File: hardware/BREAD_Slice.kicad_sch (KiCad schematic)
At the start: 15 parts, among them J1 Conn_01x10_Female, U1 AP63205

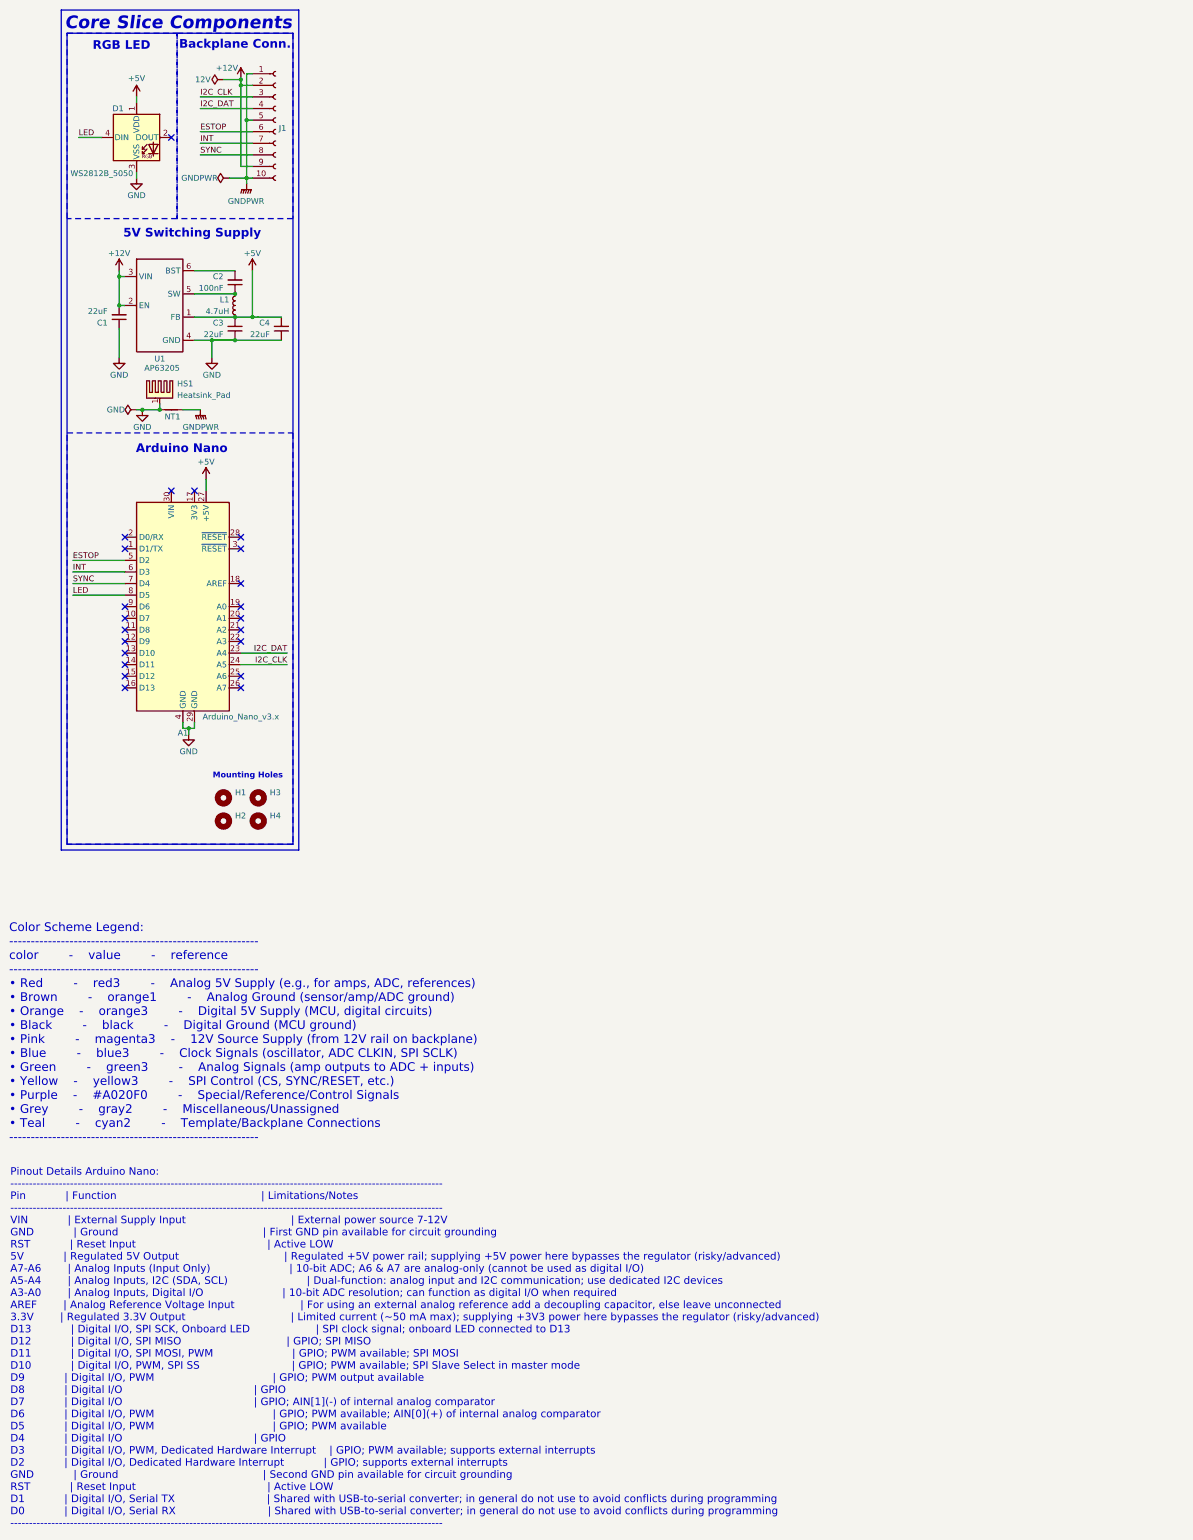
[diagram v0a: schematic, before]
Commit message: initial commit post-fork to r2
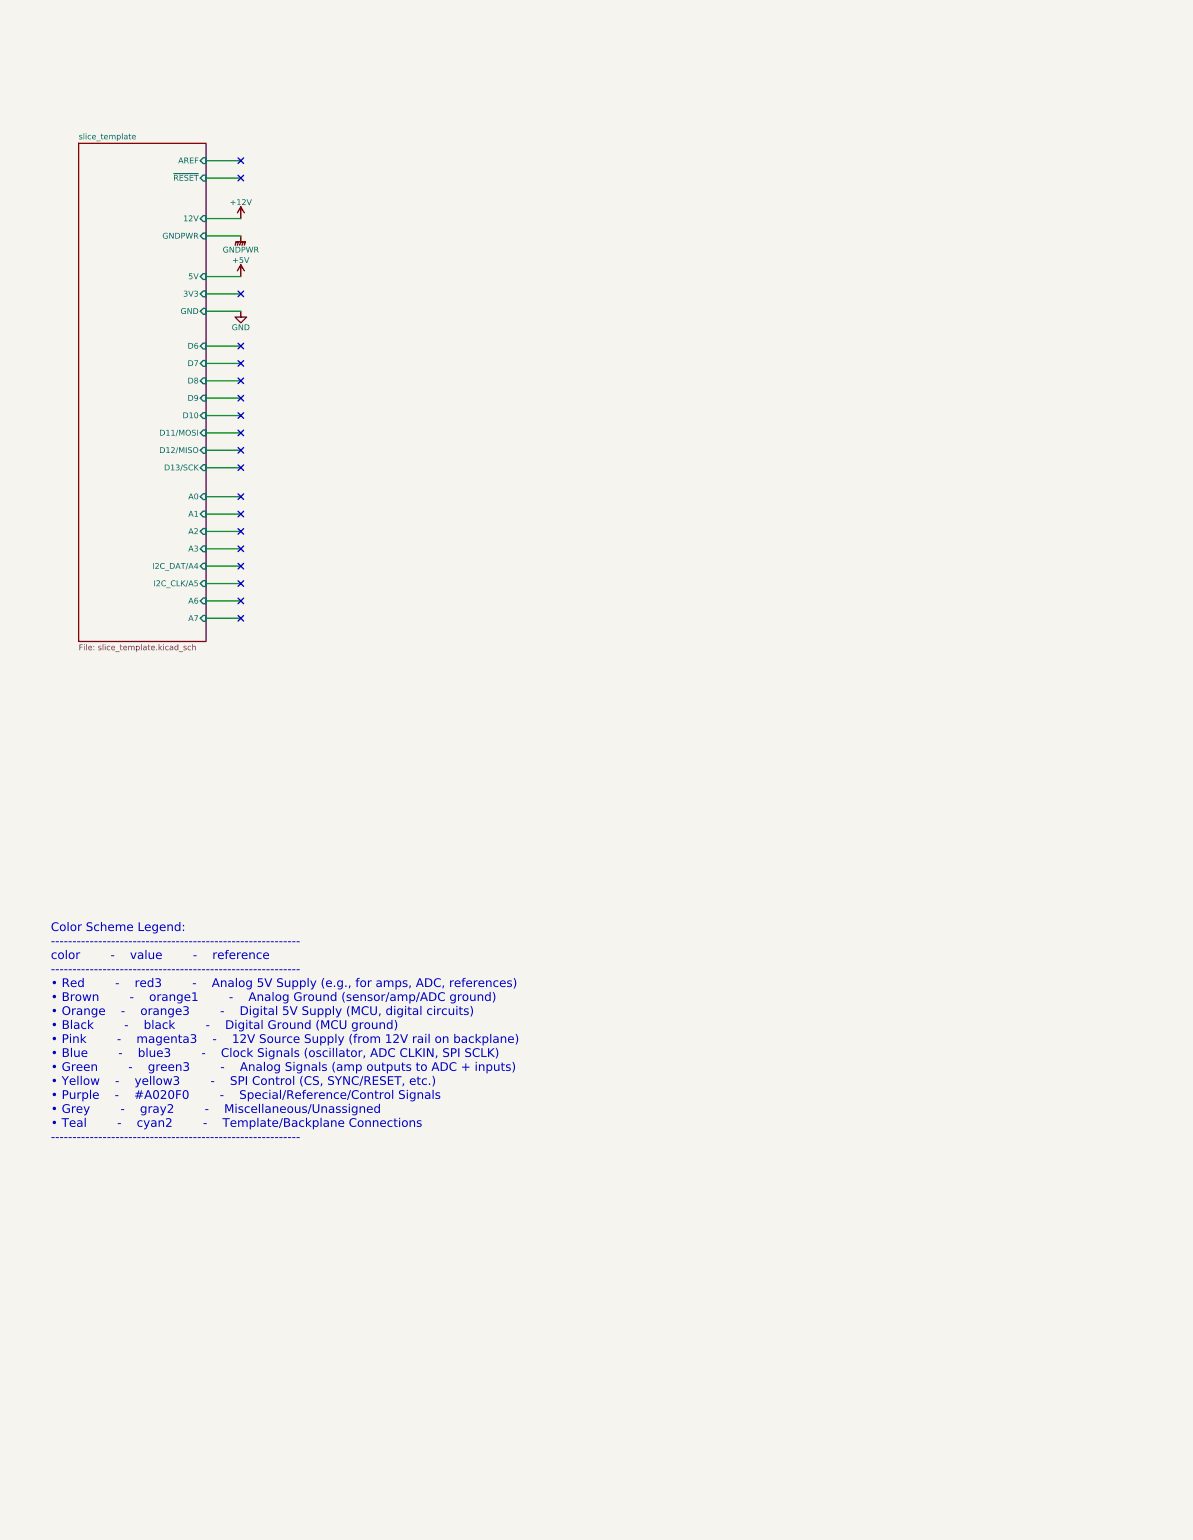
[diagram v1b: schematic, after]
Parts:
- removed A1: Arduino_Nano_v3.x, Module:Arduino_Nano, symbol MCU_Module:Arduino_Nano_v3.x
- removed C1, C3, C4: 22uF, Capacitor_SMD:C_1206_3216Metric, symbol Device:C_Small
- removed C2: 100nF, Capacitor_SMD:C_1206_3216Metric, symbol Device:C_Small
- removed D1: WS2812B_5050, SparkFun-LED:WS2812-5050-4PIN, symbol SparkFun-LED:WS2812B_5050
- removed H1, H2, H3, H4: MountingHole, MountingHole:MountingHole_5mm, symbol Mechanical:MountingHole
- removed HS1: Heatsink_Pad, kml-custom:Thermal Pad, symbol Mechanical:Heatsink_Pad
- removed J1: Conn_01x10_Female, Connector_PinSocket_2.54mm:PinSocket_1x10_P2.54mm_Horizontal, symbol Connector:Conn_01x10_Female
- removed L1: 4.7uH, Inductor_SMD:L_1210_3225Metric, symbol Device:L_Small
- removed NT1: NetTie_2, NetTie:NetTie-2_SMD_Pad2.0mm, symbol Device:NetTie_2
- removed U1: AP63205, Package_TO_SOT_SMD:TSOT-23-6, symbol SparkFun-DiscreteSemi:AP63205
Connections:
- no-connect marks 22 -> 19
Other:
- added sheet slice_template (slice_template.kicad_sch)
- note removed: "5V Switching Supply"
- note removed: "Arduino Nano"
- note removed: "Backplane Conn."
- note removed: "Core Slice Components"
- note removed: "Mounting Holes"
- note removed: "Pinout Details Arduino Nano: -------------------------------------------------------------------------------------------------------------------- Pin | Function | Limitations/Notes -------------------------------------------------------------------------------------------------------------------- VIN | External Supply Input | External power source 7-12V GND | Ground | First GND pin available for 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"
- note removed: "RGB LED"
